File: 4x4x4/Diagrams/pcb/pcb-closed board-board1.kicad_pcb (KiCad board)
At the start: 2 copper layers, 87.6 x 110.5 mm, 77 parts, among them J1 DB128V-5_0-4P, J10 DB128V-5_0-4P, J11 DB128V-5_0-4P, J12 DB128V-5_0-4P, J13 DB128V-5_0-4P, J14 DB128V-5_0-4P, J2 DB128V-5_0-6P, J3 DB128V-5_0-4P, J4 DB128V-5_0-4P, J5 DB128V-5_0-4P, J6 DB128V-5_0-4P, J7 DB128V-5_0-4P, J8 DB128V-5_0-4P, J9 DB128V-5_0-4P, Q1 2N2222, Q2 2N2222, Q3 2N2222, Q4 2N2222, U1 74HC595D,118, U2 74HC595D,118, U3 74HC595D,118, U4 74HC595D,118, U5 74HC595D,118, U6 locked, U7 74HC595D,118

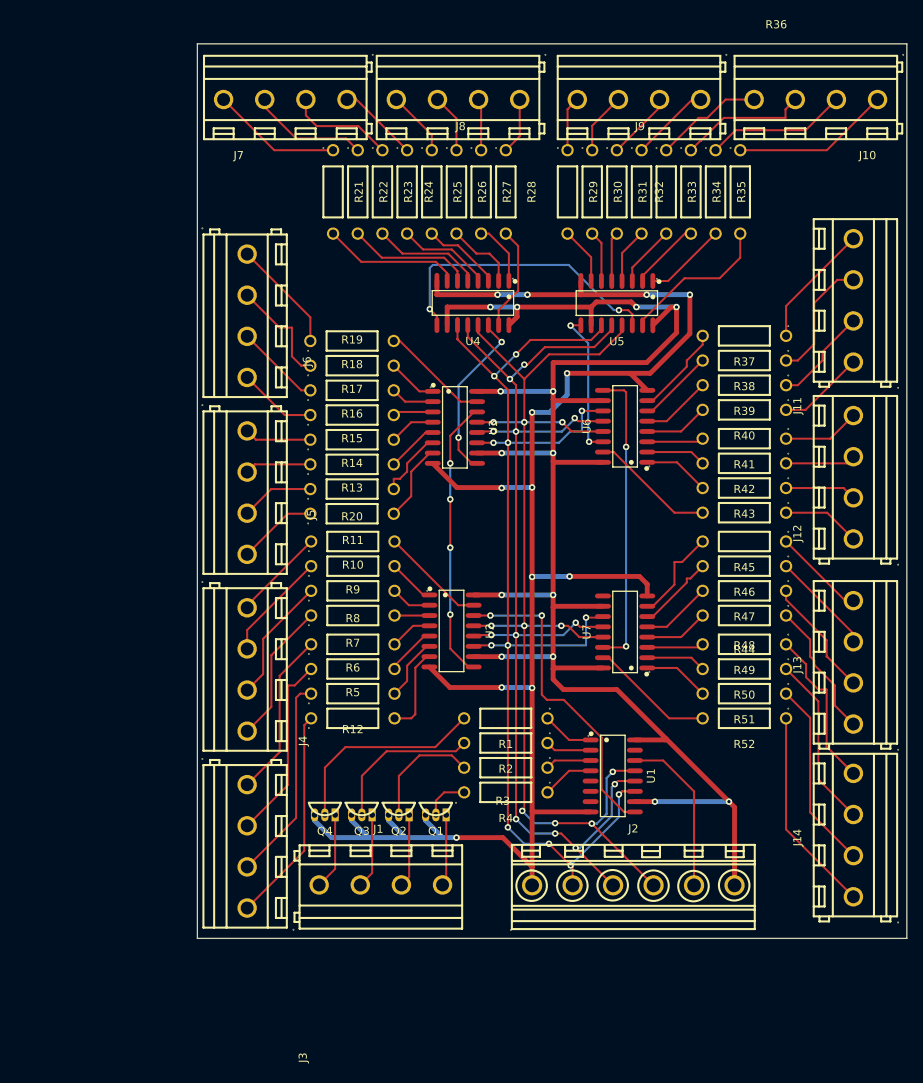
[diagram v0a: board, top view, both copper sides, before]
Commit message: create new board
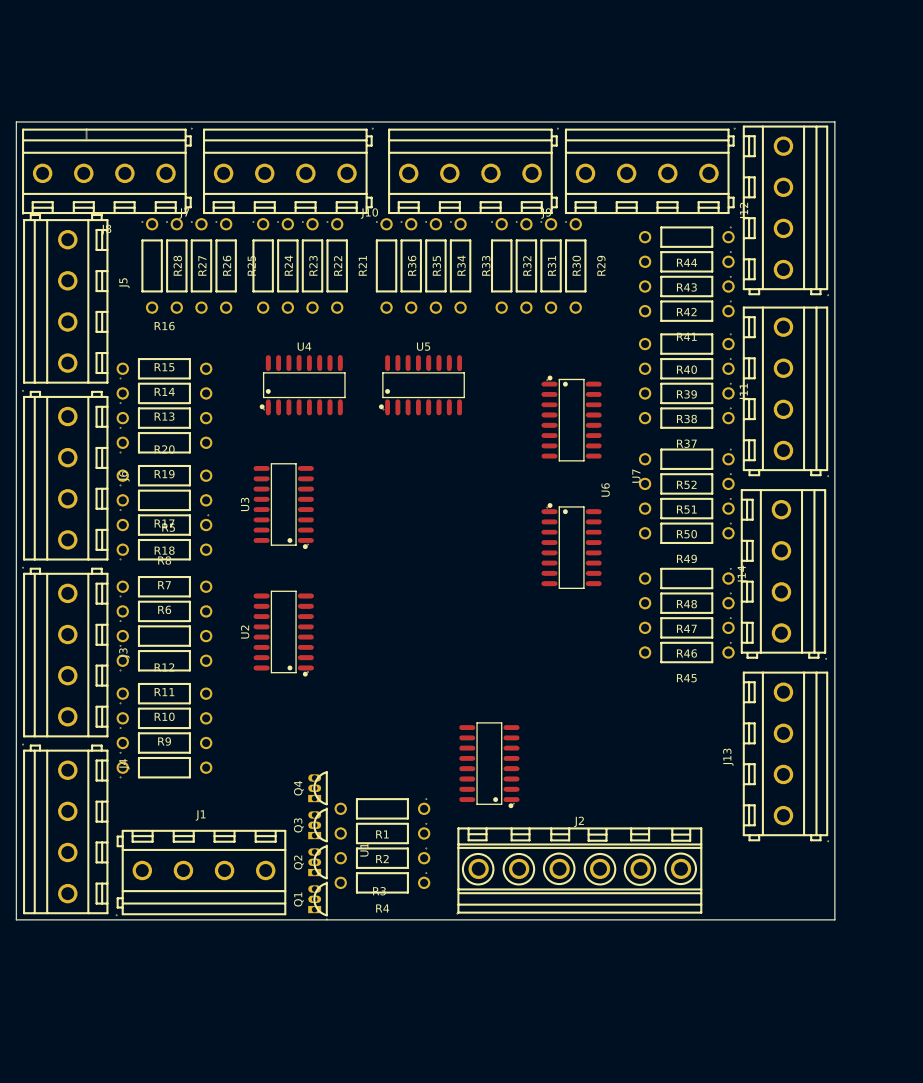
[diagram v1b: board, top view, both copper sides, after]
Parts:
- U6: value locked -> 74HC595D,118
- moved R28 44.6 mm to (48.3, 76.8)
- moved R36 44.6 mm to (77.3, 76.8)
- moved J8 44.6 mm to (42.7, 65.1)
- moved J10 43.6 mm to (87.9, 65.1)
- moved R27 38.7 mm to (51.4, 76.8)
- moved R35 38.7 mm to (80.3, 76.8)
- moved R44 34.8 mm to (114.4, 73.3)
- moved J12 34.4 mm to (126.5, 70.0)
- moved J14 33.8 mm to (126.3, 114.8)
- moved R34 32.8 mm to (83.4, 76.8)
- moved R26 32.8 mm to (54.4, 76.8)
- moved R52 32.8 mm to (114.4, 100.7)
- moved J3 32.4 mm to (37.6, 124.6)
- moved J5 32.4 mm to (37.6, 80.9)
- moved R11 29.9 mm to (49.8, 132.7)
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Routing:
- net GND: track 217.6 -> 0.00 mm, vias 13 -> 0
- net Net-(J2-Pad6): track 216.3 -> 0.00 mm, vias 14 -> 0
- net Net-(J2-Pad2): track 144.6 -> 1.20 mm, vias 12 -> 0
- net Net-(J2-Pad3): track 140.7 -> 0.00 mm, vias 12 -> 0
- net Net-(J2-Pad4): track 140.0 -> 0.00 mm, vias 10 -> 0
- net Net-(U1-Pad9): track 39.4 -> 0.00 mm, vias 2 -> 0
- net Net-(U6-Pad9): track 37.3 -> 0.00 mm, vias 2 -> 0
- net Net-(U4-Pad9): track 36.5 -> 0.00 mm, vias 2 -> 0
- net Net-(U2-Pad9): track 34.6 -> 0.00 mm, vias 4 -> 0
- net Net-(J3-Pad4): track 26.7 -> 0.00 mm
- net Net-(Q4-Pad2): track 25.6 -> 0.00 mm
- net Net-(J14-Pad1): track 25.5 -> 0.00 mm
- net Net-(J3-Pad3): track 25.5 -> 0.00 mm
- net Net-(J14-Pad2): track 23.5 -> 0.00 mm
- net Net-(J3-Pad2): track 23.1 -> 0.00 mm
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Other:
- board size 87.6 x 110.5 mm -> 101.1 x 98.6 mm
